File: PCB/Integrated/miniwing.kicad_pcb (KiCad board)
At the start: 2 copper layers, 184.6 x 86.5 mm, 69 parts, among them U1 rp2040-zero

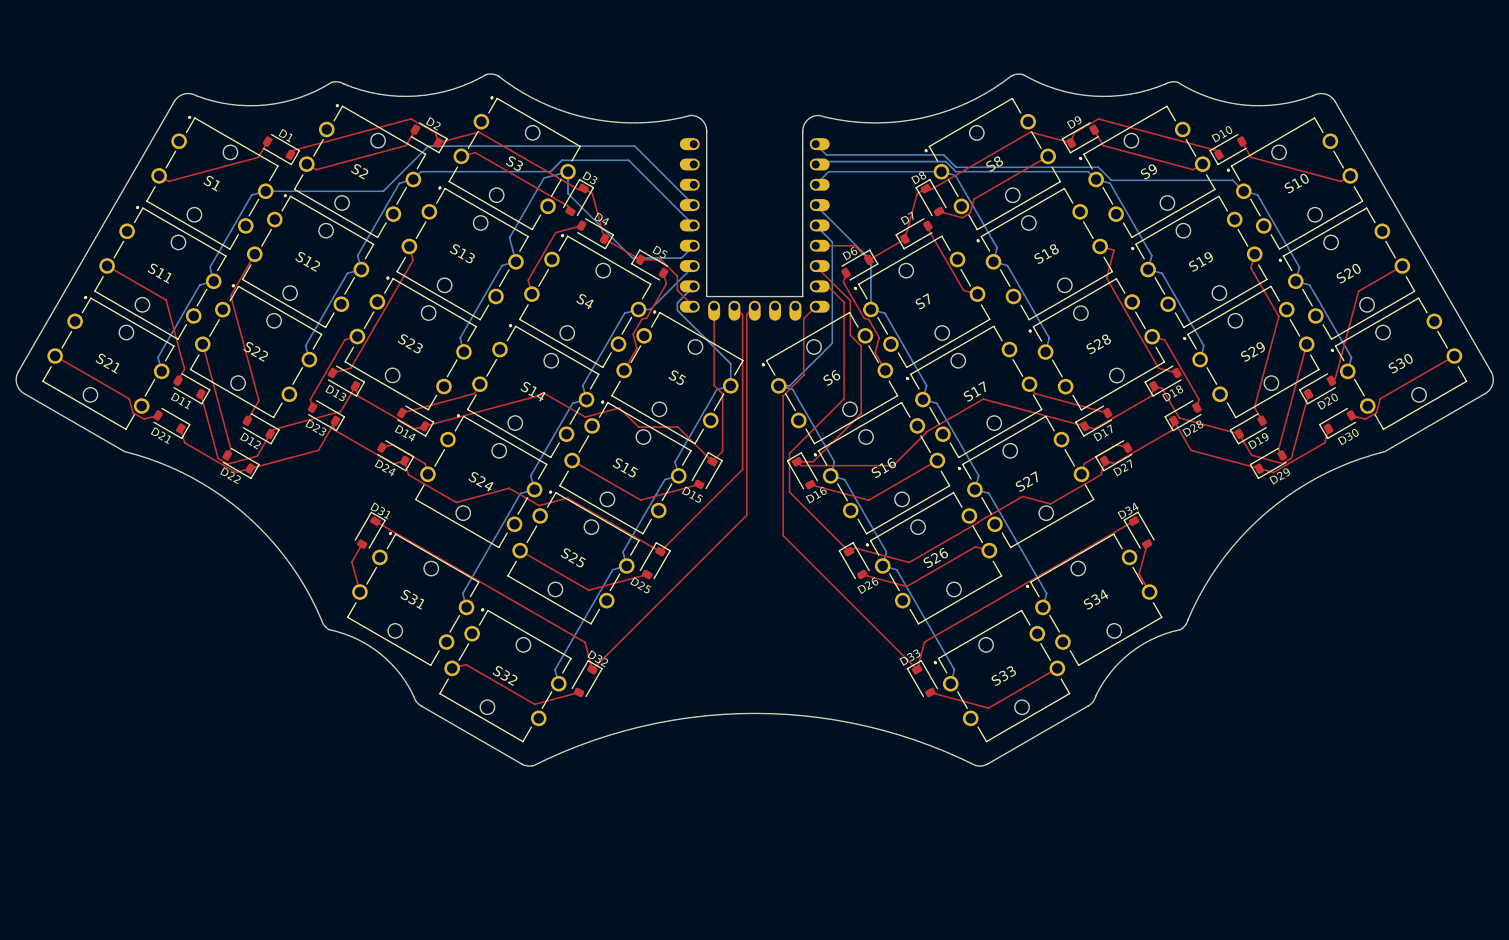
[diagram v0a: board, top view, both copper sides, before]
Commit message: Hopefully complete first version of integrated pcb.
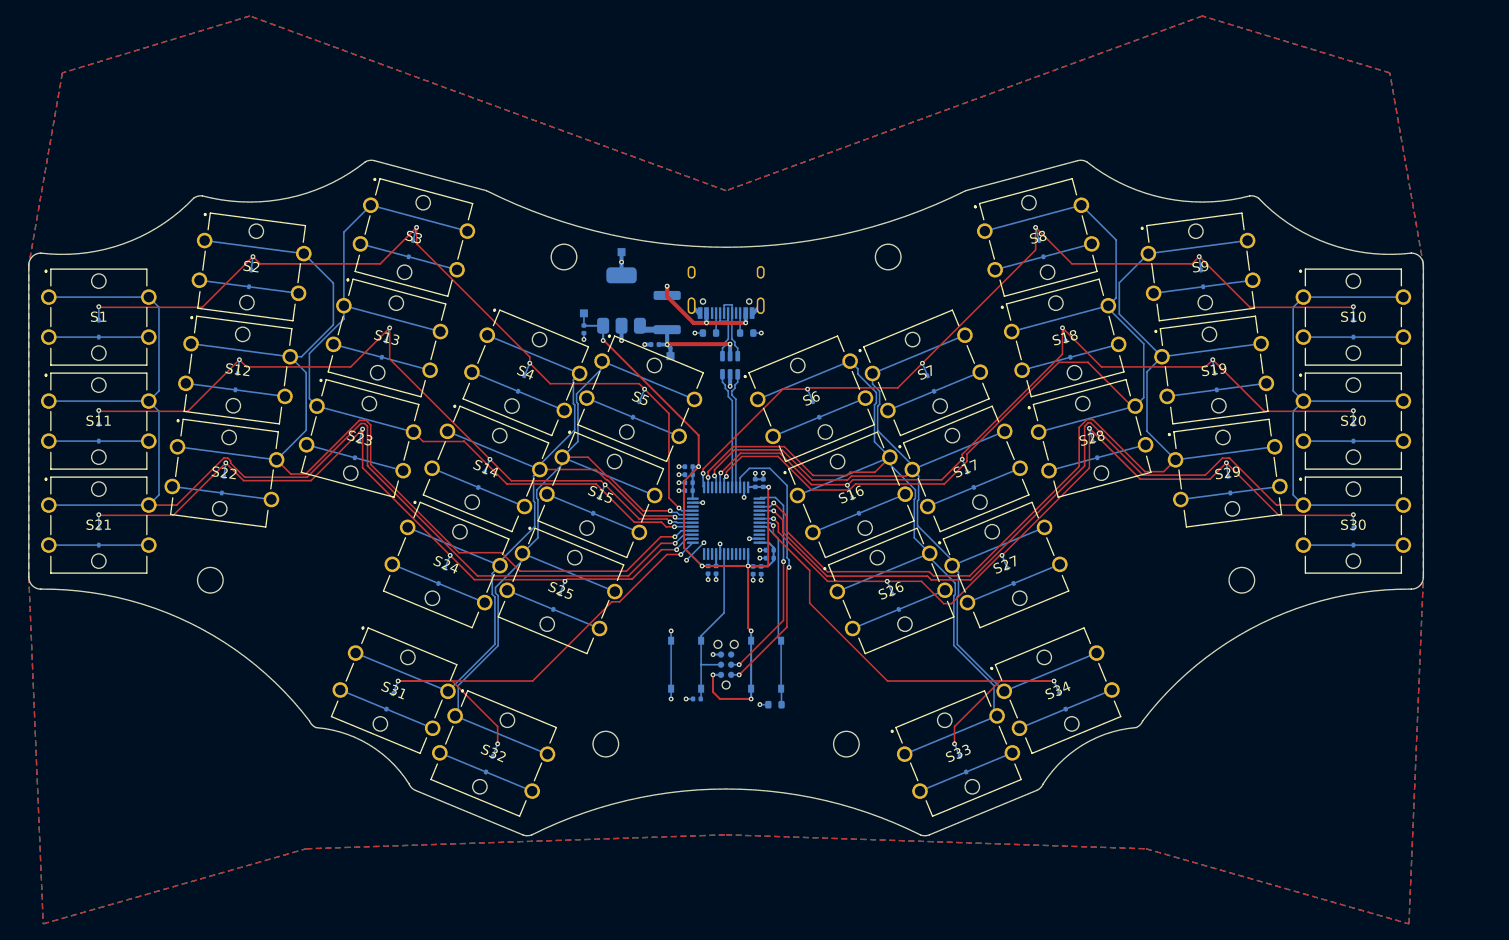
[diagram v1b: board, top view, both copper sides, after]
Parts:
- added BOOT1: SW_Push, Button_Switch_SMD:SW_Push_1P1T_XKB_TS-1187A, B.Cu at (154.9, 110.3)
- added C1: 10nF, Capacitor_SMD:C_0402_1005Metric, B.Cu at (147.6, 98.5)
- added C10: 4.7uF, Capacitor_SMD:C_0402_1005Metric, B.Cu at (153.2, 98.5)
- added C11: 100nF, Capacitor_SMD:C_0402_1005Metric, B.Cu at (145.2, 88.6)
- added C12: 100nF, Capacitor_SMD:C_0402_1005Metric, B.Cu at (145.2, 87.6)
- added C13: 100nF, Capacitor_SMD:C_0402_1005Metric, B.Cu at (145.2, 86.6)
- added C14: 4.7uF, Capacitor_SMD:C_0402_1005Metric, B.Cu at (145.2, 85.6)
- added C15: 100nF, Capacitor_SMD:C_0402_1005Metric, B.Cu at (146.2, 114.6)
- added C2: 1uF, Capacitor_SMD:C_0402_1005Metric, B.Cu at (148.6, 98.5)
- added C3: 100nF, Capacitor_SMD:C_0402_1005Metric, B.Cu at (154.5, 87.6)
- added C4: 4.7uF, Capacitor_SMD:C_0402_1005Metric, B.Cu at (153.5, 87.6)
- added C5: 1uF, Capacitor_SMD:C_0402_1005Metric, B.Cu at (141.0, 70.3)
- added C6: 1uF, Capacitor_SMD:C_0402_1005Metric, B.Cu at (132.1, 68.4)
- added C7: 100nF, Capacitor_SMD:C_0402_1005Metric, B.Cu at (155.3, 97.0)
- added C8: 100nF, Capacitor_SMD:C_0402_1005Metric, B.Cu at (155.3, 96.0)
- added C9: 100nF, Capacitor_SMD:C_0402_1005Metric, B.Cu at (154.2, 98.5)
- added F1: Polyfuse_Small, Fuse:Fuse_1812_4532Metric, B.Cu at (142.5, 66.3)
- added H1: MountingHole, MountingHole:MountingHole_3.2mm_M3, B.Cu at (129.6, 59.4)
- added H2: MountingHole, MountingHole:MountingHole_3.2mm_M3, B.Cu at (170.1, 59.4)
- added H3: MountingHole, MountingHole:MountingHole_3.2mm_M3, B.Cu at (214.3, 99.8)
- added H4: MountingHole, MountingHole:MountingHole_3.2mm_M3, B.Cu at (164.9, 120.2)
- added H5: MountingHole, MountingHole:MountingHole_3.2mm_M3, B.Cu at (134.8, 120.2)
- added H6: MountingHole, MountingHole:MountingHole_3.2mm_M3, B.Cu at (85.4, 99.8)
- added J1: USB_C_Receptacle_USB2.0_16P, Connector_USB:USB_C_Receptacle_HRO_TYPE-C-31-M-12, B.Cu at (149.9, 62.3)
- added J3: Conn_ARM_SWD_TagConnect_TC2030-NL, Connector:Tag-Connect_TC2030-IDC-NL_2x03_P1.27mm_Vertical, B.Cu at (149.9, 110.3)
- added R1: 10k, Resistor_SMD:R_0603_1608Metric, B.Cu at (156.0, 115.3)
- added R2: 5.1k, Resistor_SMD:R_0603_1608Metric, B.Cu at (147.8, 68.9)
- added R3: 5.1k, Resistor_SMD:R_0603_1608Metric, B.Cu at (152.4, 68.9)
- added RESET1: SW_Push, Button_Switch_SMD:SW_Push_1P1T_XKB_TS-1187A, B.Cu at (144.9, 110.3)
- added TP1: TestPoint_Alt, TestPoint:TestPoint_Pad_1.0x1.0mm, B.Cu at (132.1, 66.4)
- added TP2: TestPoint_Alt, TestPoint:TestPoint_Pad_1.0x1.0mm, B.Cu at (142.9, 71.7)
- added TP3: TestPoint_Alt, TestPoint:TestPoint_Pad_1.0x1.0mm, B.Cu at (136.8, 58.8)
- added U2: USBLC6-2SC6, Package_TO_SOT_SMD:SOT-23-6, B.Cu at (150.4, 72.9)
- added U3: STM32F072CBTx, Package_QFP:LQFP-48_7x7mm_P0.5mm, B.Cu at (149.9, 92.3)
- D1, D10, D11, D12, D13, D14, D15, D16, D17, D18, D19, D2, D20, D21, D22, D23, D24, D25, D26, D27, D28, D29, D3, D30, D31, D32, D33, D34, D4, D5, D6, D7, D8, D9: value D_Small -> 1N4148; footprint Diode_SMD:D_SOD-123 -> Diode_SMD:D_SOD-323; moved to B.Cu
- U1: value rp2040-zero -> TC1262-33; footprint mcu:rp2040-zero-tht -> Package_TO_SOT_SMD:SOT-223-3_TabPin2; moved to B.Cu
- moved D1 31.9 mm to (71.5, 68.3), turned to -90 degrees
- moved D2 28.3 mm to (90.4, 62.0), turned to -97.5 degrees
- moved D10 27.3 mm to (228.3, 68.3), turned to -90 degrees
- moved D34 23.2 mm to (191.9, 114.9), turned to -67.5 degrees
- moved D9 23.2 mm to (209.4, 62.0), turned to -82.5 degrees
- moved S1 21.9 mm to (71.5, 66.9), turned to 0 degrees
- moved D3 21.6 mm to (110.5, 58.3), turned to -105 degrees
- moved D31 21.2 mm to (107.8, 114.9), turned to -112.5 degrees
- moved S30 21.0 mm to (228.3, 92.9), turned to 0 degrees
- moved D4 20.9 mm to (124.3, 75.2), turned to -112.5 degrees
- moved S21 20.2 mm to (71.5, 92.9), turned to 0 degrees
- moved D27 20.1 mm to (185.4, 99.2), turned to -67.5 degrees
- moved S11 20.0 mm to (71.5, 79.9), turned to 0 degrees
- moved U1 19.1 mm to (136.8, 64.8), turned to 90 degrees
- moved D7 19.0 mm to (175.5, 75.2), turned to -67.5 degrees
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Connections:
- S1 pad 1: unconnected-(S1-NO_1-Pad1) -> COL-00
- S1 pad 4: unconnected-(S1-NO_4-Pad4) -> Net-(D1-A)
- S10 pad 2: unconnected-(S10-NO_2-Pad2) -> COL-10
- S10 pad 3: unconnected-(S10-NO_3-Pad3) -> Net-(D10-A)
- S11 pad 1: unconnected-(S11-NO_1-Pad1) -> COL-00
- S11 pad 4: unconnected-(S11-NO_4-Pad4) -> Net-(D11-A)
- S12 pad 1: unconnected-(S12-NO_1-Pad1) -> COL-01
- S12 pad 4: unconnected-(S12-NO_4-Pad4) -> Net-(D12-A)
- S13 pad 1: unconnected-(S13-NO_1-Pad1) -> COL-02
- S13 pad 4: unconnected-(S13-NO_4-Pad4) -> Net-(D13-A)
- S14 pad 1: unconnected-(S14-NO_1-Pad1) -> COL-03
- S14 pad 4: unconnected-(S14-NO_4-Pad4) -> Net-(D14-A)
- S15 pad 1: unconnected-(S15-NO_1-Pad1) -> COL-04
- S15 pad 4: unconnected-(S15-NO_4-Pad4) -> Net-(D15-A)
- S16 pad 2: unconnected-(S16-NO_2-Pad2) -> COL-14
- S16 pad 3: unconnected-(S16-NO_3-Pad3) -> Net-(D16-A)
- S17 pad 2: unconnected-(S17-NO_2-Pad2) -> COL-13
- S17 pad 3: unconnected-(S17-NO_3-Pad3) -> Net-(D17-A)
- S18 pad 2: unconnected-(S18-NO_2-Pad2) -> COL-12
- S18 pad 3: unconnected-(S18-NO_3-Pad3) -> Net-(D18-A)
- S19 pad 2: unconnected-(S19-NO_2-Pad2) -> COL-11
- S19 pad 3: unconnected-(S19-NO_3-Pad3) -> Net-(D19-A)
- S2 pad 1: unconnected-(S2-NO_1-Pad1) -> COL-01
- S2 pad 4: unconnected-(S2-NO_4-Pad4) -> Net-(D2-A)
- S20 pad 2: unconnected-(S20-NO_2-Pad2) -> COL-10
- S20 pad 3: unconnected-(S20-NO_3-Pad3) -> Net-(D20-A)
- S21 pad 1: unconnected-(S21-NO_1-Pad1) -> COL-00
- S21 pad 4: unconnected-(S21-NO_4-Pad4) -> Net-(D21-A)
- S22 pad 1: unconnected-(S22-NO_1-Pad1) -> COL-01
- S22 pad 4: unconnected-(S22-NO_4-Pad4) -> Net-(D22-A)
- S23 pad 1: unconnected-(S23-NO_1-Pad1) -> COL-02
- S23 pad 4: unconnected-(S23-NO_4-Pad4) -> Net-(D23-A)
- S24 pad 1: unconnected-(S24-NO_1-Pad1) -> COL-03
- S24 pad 4: unconnected-(S24-NO_4-Pad4) -> Net-(D24-A)
- S25 pad 1: unconnected-(S25-NO_1-Pad1) -> COL-04
- S25 pad 4: unconnected-(S25-NO_4-Pad4) -> Net-(D25-A)
- S26 pad 2: unconnected-(S26-NO_2-Pad2) -> COL-14
- S26 pad 3: unconnected-(S26-NO_3-Pad3) -> Net-(D26-A)
- S27 pad 2: unconnected-(S27-NO_2-Pad2) -> COL-13
- S27 pad 3: unconnected-(S27-NO_3-Pad3) -> Net-(D27-A)
- S28 pad 2: unconnected-(S28-NO_2-Pad2) -> COL-12
- S28 pad 3: unconnected-(S28-NO_3-Pad3) -> Net-(D28-A)
- S29 pad 2: unconnected-(S29-NO_2-Pad2) -> COL-11
- S29 pad 3: unconnected-(S29-NO_3-Pad3) -> Net-(D29-A)
- S3 pad 1: unconnected-(S3-NO_1-Pad1) -> COL-02
- S3 pad 4: unconnected-(S3-NO_4-Pad4) -> Net-(D3-A)
- S30 pad 2: unconnected-(S30-NO_2-Pad2) -> COL-10
- S30 pad 3: unconnected-(S30-NO_3-Pad3) -> Net-(D30-A)
- S31 pad 1: unconnected-(S31-NO_1-Pad1) -> COL-03
- S31 pad 4: unconnected-(S31-NO_4-Pad4) -> Net-(D31-A)
- S32 pad 1: unconnected-(S32-NO_1-Pad1) -> COL-04
- S32 pad 4: unconnected-(S32-NO_4-Pad4) -> Net-(D32-A)
- S33 pad 2: unconnected-(S33-NO_2-Pad2) -> COL-14
- S33 pad 3: unconnected-(S33-NO_3-Pad3) -> Net-(D33-A)
- S34 pad 2: unconnected-(S34-NO_2-Pad2) -> COL-13
- S34 pad 3: unconnected-(S34-NO_3-Pad3) -> Net-(D34-A)
- S4 pad 1: unconnected-(S4-NO_1-Pad1) -> COL-03
- S4 pad 4: unconnected-(S4-NO_4-Pad4) -> Net-(D4-A)
- S5 pad 1: unconnected-(S5-NO_1-Pad1) -> COL-04
- S5 pad 4: unconnected-(S5-NO_4-Pad4) -> Net-(D5-A)
- S6 pad 2: unconnected-(S6-NO_2-Pad2) -> COL-14
- S6 pad 3: unconnected-(S6-NO_3-Pad3) -> Net-(D6-A)
- S7 pad 2: unconnected-(S7-NO_2-Pad2) -> COL-13
- S7 pad 3: unconnected-(S7-NO_3-Pad3) -> Net-(D7-A)
- S8 pad 2: unconnected-(S8-NO_2-Pad2) -> COL-12
- S8 pad 3: unconnected-(S8-NO_3-Pad3) -> Net-(D8-A)
- S9 pad 2: unconnected-(S9-NO_2-Pad2) -> COL-11
- S9 pad 3: unconnected-(S9-NO_3-Pad3) -> Net-(D9-A)
- U1 pad 1: COL-10 -> +5V
- U1 pad 2: COL-11 -> GND
- U1 pad 3: COL-12 -> VDD
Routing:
- net VDD: track 0.00 -> 103.3 mm, vias 0 -> 8
- net COL-12: track 44.5 -> 94.7 mm, vias 0 -> 1
- net GND: track 0.00 -> 42.3 mm, vias 0 -> 30
- net ROW-10: track 60.7 -> 102.7 mm, vias 0 -> 6
- net COL-11: track 64.2 -> 103.1 mm, vias 0 -> 1
- net ROW-00: track 63.5 -> 101.7 mm, vias 0 -> 6
- net SWD_IO: track 0.00 -> 35.8 mm, vias 0 -> 2
- net COL-10: track 84.1 -> 117.6 mm, vias 0 -> 1
- net COL-01: track 67.5 -> 101.0 mm, vias 0 -> 1
- net COL-00: track 87.0 -> 115.4 mm, vias 0 -> 1
- net SWD_CLK: track 0.00 -> 26.7 mm, vias 0 -> 2
- net ROW-03: track 87.6 -> 61.0 mm, vias 0 -> 3
- net BOOT0: track 0.00 -> 23.9 mm
- net ROW-13: track 87.8 -> 65.0 mm, vias 0 -> 3
- net Net-(D19-A): track 22.5 -> 0.00 mm
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- added copper zone on B.Cu, net GND
- added copper zone on F.Cu, net GND
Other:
- board size 184.6 x 86.5 mm -> 174.3 x 84.4 mm
